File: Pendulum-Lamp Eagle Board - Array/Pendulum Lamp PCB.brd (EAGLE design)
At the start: 121.9 x 33 mm, 25 parts, among them U1 QRD1114, U2 QRD1114, U3 QRD1114, U4 QRD1114, U5 QRD1114, U6 QRD1114, U7 QRD1114, U8 QRD1114, X2 2514-

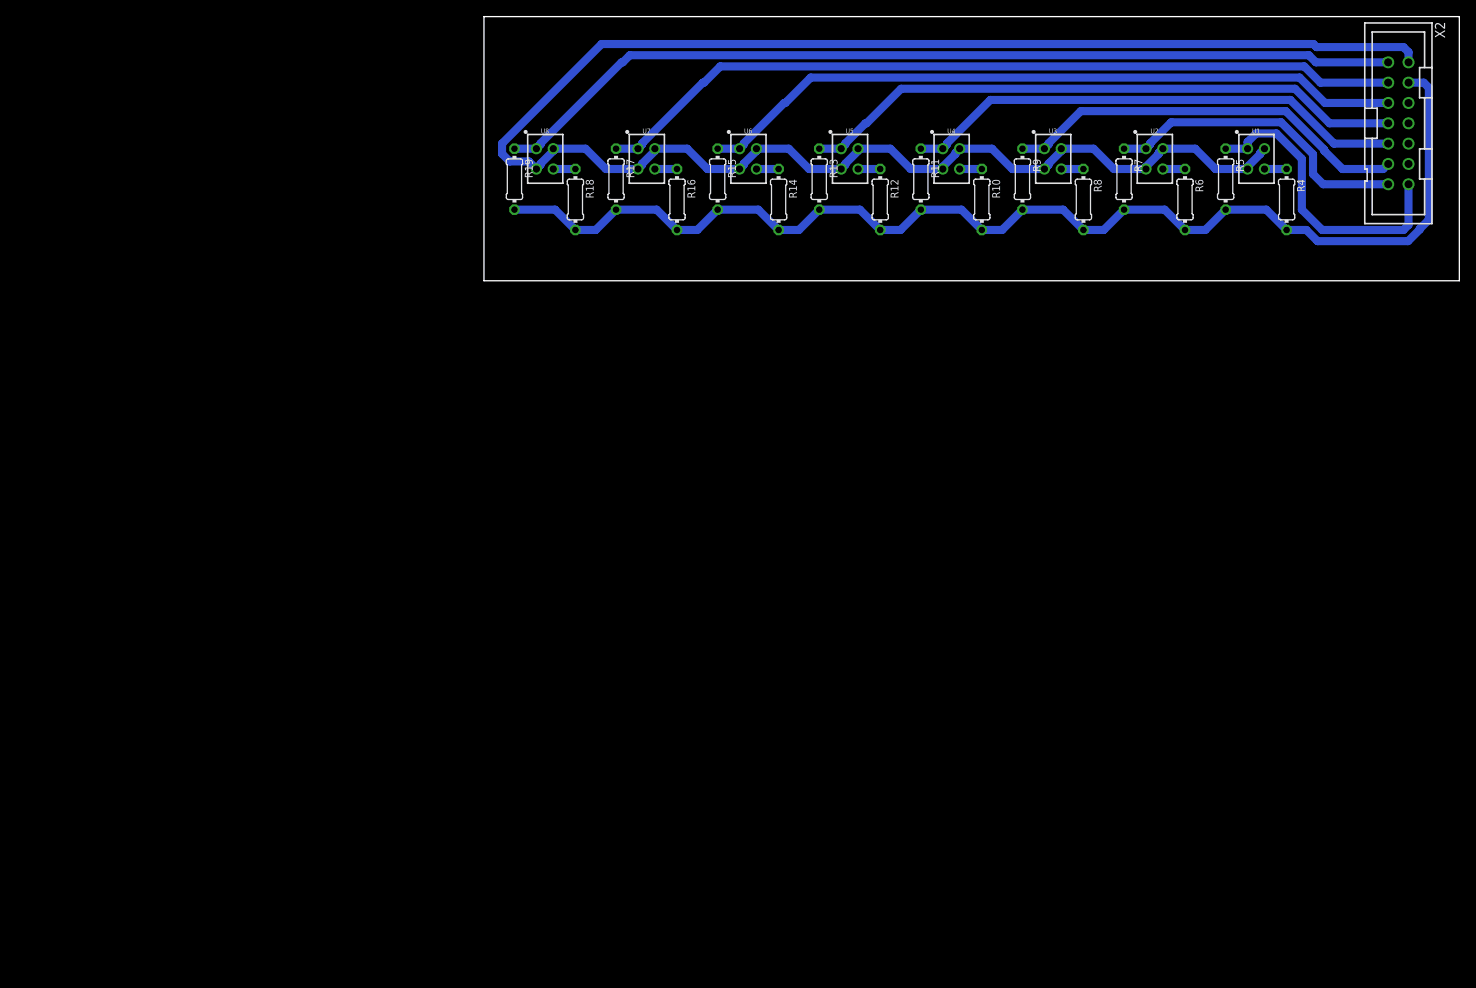
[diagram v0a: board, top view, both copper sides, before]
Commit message: First succesful model
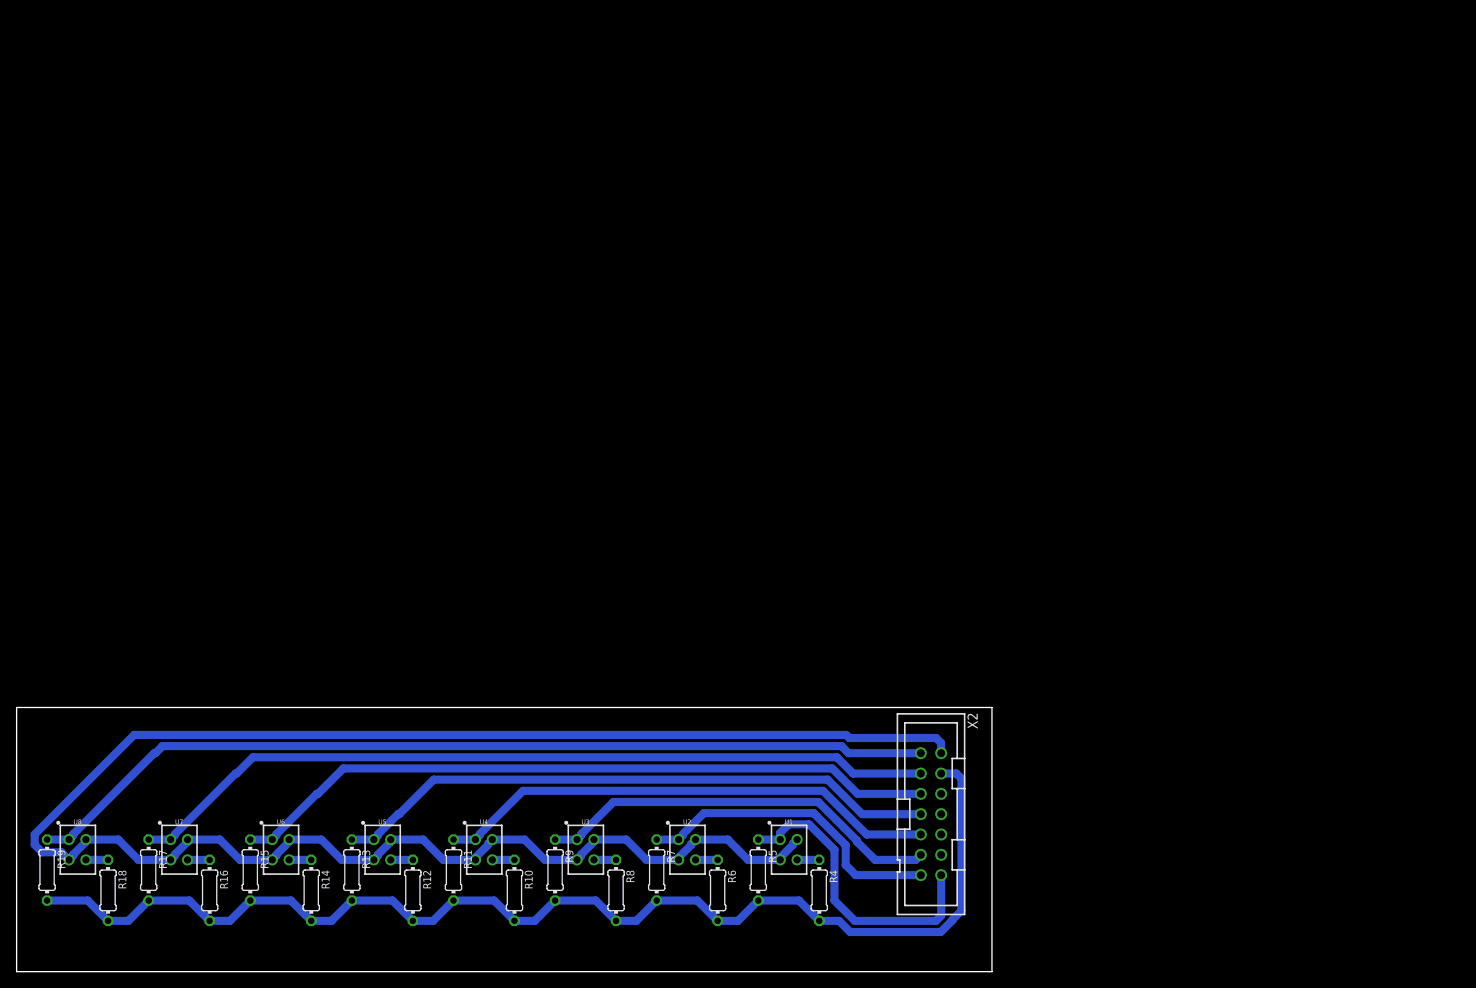
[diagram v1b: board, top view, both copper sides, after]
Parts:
- moved R10 104.3 mm to (62.2, 10.8)
- moved R12 104.3 mm to (49.5, 10.8)
- moved R14 104.3 mm to (36.8, 10.8)
- moved R16 104.3 mm to (24.1, 10.8)
- moved R4 104.3 mm to (100.3, 10.8)
- moved R6 104.3 mm to (87.6, 10.8)
- moved U1 104.3 mm to (96.5, 15.9)
- moved U2 104.3 mm to (83.8, 15.9)
- moved U4 104.3 mm to (58.4, 15.9)
- moved U5 104.3 mm to (45.7, 15.9)
- moved U8 104.3 mm to (7.62, 15.9)
- moved X2 104.3 mm to (114.3, 20.3)
- moved R11 104.3 mm to (54.6, 13.3)
- moved R13 104.3 mm to (41.9, 13.3)
- moved R15 104.3 mm to (29.2, 13.3)
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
